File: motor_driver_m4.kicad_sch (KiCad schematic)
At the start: 32 parts, among them J13 Conn_01x01_Pin, J14 Conn_01x01_Pin, J15 Conn_01x01_Pin, M4 DRV8320SRTVR, Q19 NP80N06D6, Q20 NP80N06D6, Q21 NP80N06D6, Q22 NP80N06D6, Q23 NP80N06D6, Q24 NP80N06D6

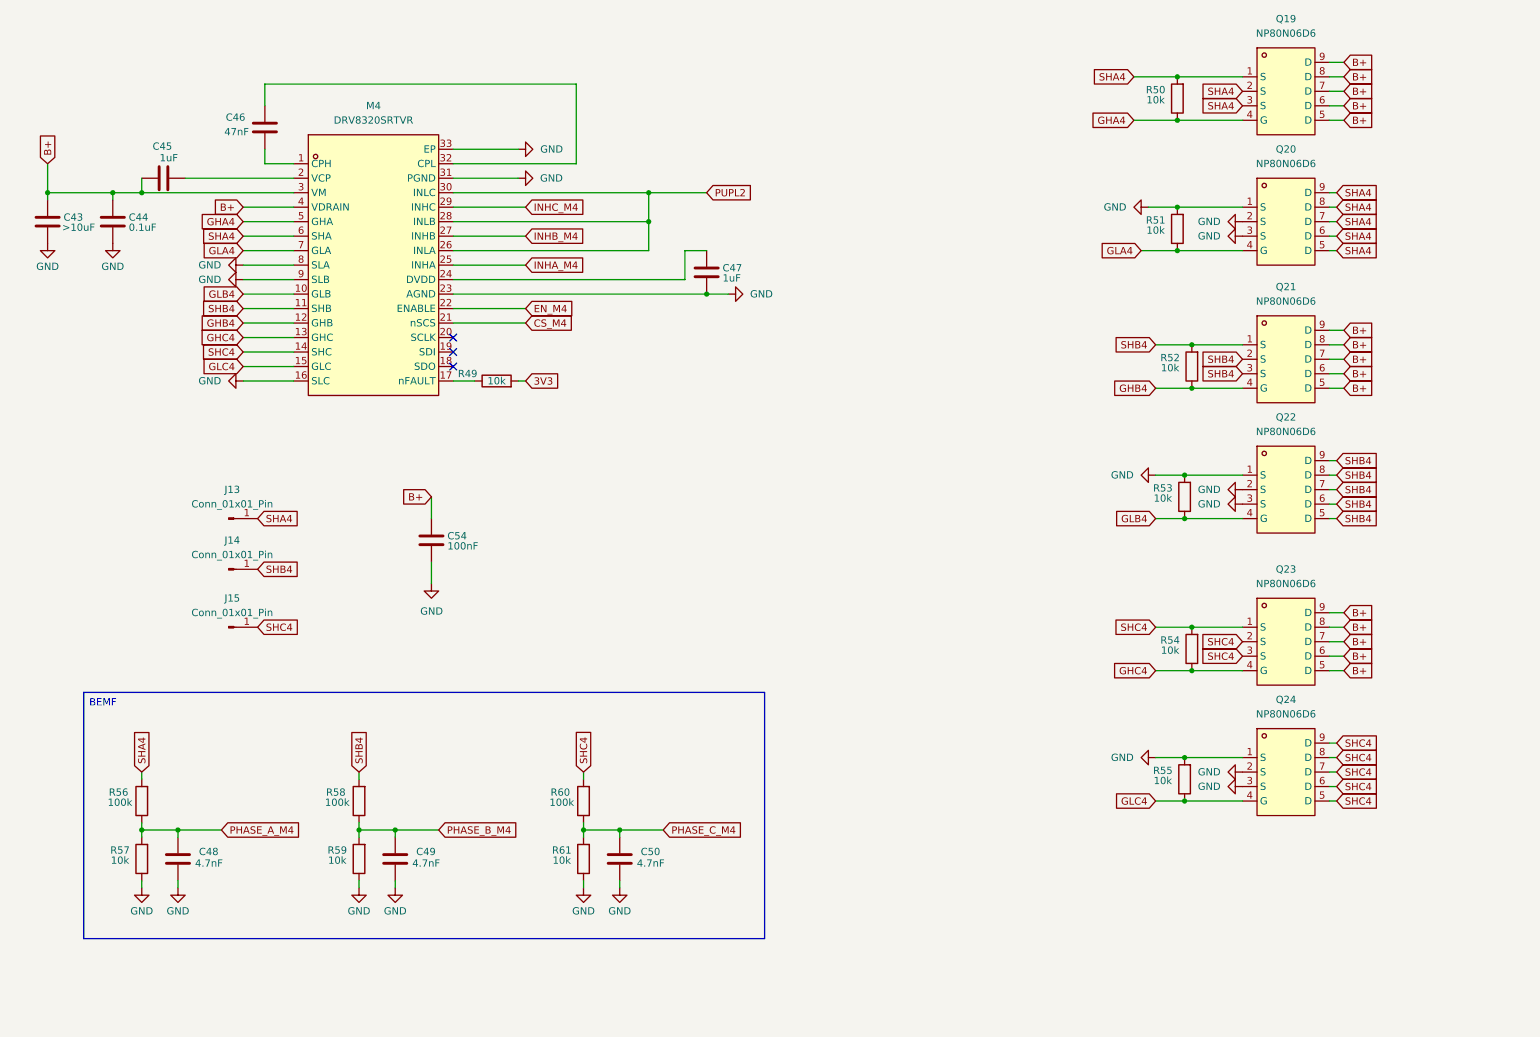
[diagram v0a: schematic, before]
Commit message: complete change in architecture,work in progress
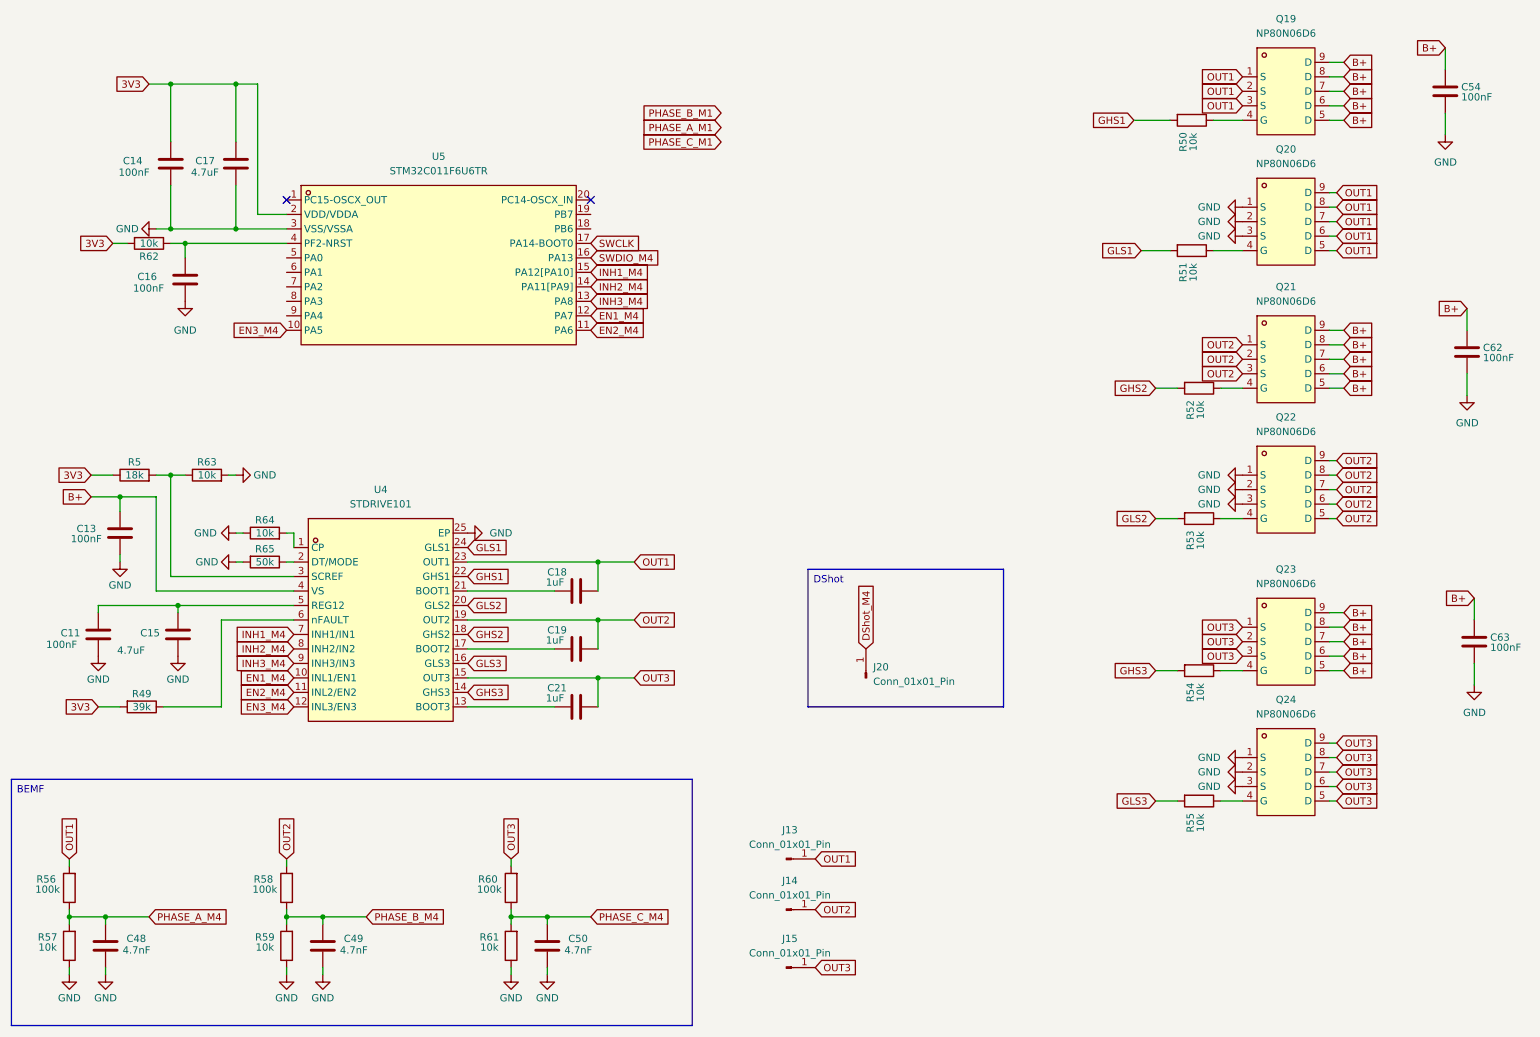
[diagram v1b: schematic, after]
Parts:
- removed C43: >10uF, easyeda2kicad:C0603, symbol Device:C
- removed C44: 0.1uF, easyeda2kicad:C0402, symbol Device:C
- removed C45, C47: 1uF, easyeda2kicad:C0603, symbol Device:C
- removed C46: 47nF, easyeda2kicad:C0603, symbol Device:C
- removed M4: DRV8320SRTVR, easyeda2kicad:WQFN-32_L5.0-W5.0-P0.50-TL-EP3.5, symbol easyeda2kicad:DRV8320SRTVR
- added C11, C62, C63: 100nF, easyeda2kicad:C0603, symbol Device:C
- added C13, C14, C16: 100nF, easyeda2kicad:C0402, symbol Device:C
- added C15: 4.7uF, easyeda2kicad:C0603, symbol Device:C
- added C17: 4.7uF, easyeda2kicad:C0402, symbol Device:C
- added C18, C19, C21: 1uF, easyeda2kicad:C0402, symbol Device:C
- added J20: Conn_01x01_Pin, deshan:Conn_1x1_small, symbol Connector:Conn_01x01_Pin
- added R5: 18k, easyeda2kicad:R0402, symbol Device:R
- added R62, R63, R64: 10k, easyeda2kicad:R0402, symbol Device:R
- added R65: 50k, easyeda2kicad:R0402, symbol Device:R
- added U4: STDRIVE101, easyeda2kicad:QFN-24_L4.0-W4.0-P0.50-BL-EP2.7, symbol easyeda2kicad:STDRIVE101
- added U5: STM32C011F6U6TR, easyeda2kicad:UFQFPN-20_L3.0-W3.0-P0.50-TL, symbol easyeda2kicad:STM32C011F6U6TR
- R49: value 10k -> 39k
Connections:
- net 3V3: now also C14.1, C17.1, R5.1, R62.2, U5.2 (VDD/VDDA)
- net B+: now also C13.1, C62.1, C63.1, U4.4 (VS)
- net GND: now also C11.2, C13.2, C14.2, C15.2, C16.2, C17.2, C62.2, C63.2, R63.2, R64.1, R65.2, U4.25 (EP), U5.3 (VSS/VSSA); no longer R51.2, R53.2, R55.2
- net at R49.1: now also U4.6 (nFAULT)
- net GHA4: no longer names the net of Q19.4 (G), R50.1
- net GHB4: no longer names the net of Q21.4 (G), R52.1
- net GHC4: no longer names the net of Q23.4 (G), R54.1
- net GLA4: no longer names the net of Q20.4 (G), R51.1
- net GLB4: no longer names the net of Q22.4 (G), R53.1
- net GLC4: no longer names the net of Q24.4 (G), R55.1
- net SHA4 renamed OUT1
- net OUT1: now also C18.1, U4.23 (OUT1); no longer R50.2
- net SHB4 renamed OUT2
- net OUT2: now also C19.1, U4.19 (OUT2); no longer R52.2
- net SHC4 renamed OUT3
- net OUT3: now also C21.1, U4.15 (OUT3); no longer R54.2
- new net: R65.1, U4.2 (DT/MODE)
- new net: C18.2, U4.21 (BOOT1)
- new net: C11.1, C15.1, U4.5 (REG12)
- new net: R64.2, U4.1 (CP)
- new net: C21.2, U4.13 (BOOT3)
- new net: C19.2, U4.17 (BOOT2)
- new net: R5.2, R63.1, U4.3 (SCREF)
- new net: C16.1, R62.1, U5.4 (PF2-NRST)
- new net DShot_M4: J20.1 (Pin_1)
- new net EN1_M4: U4.10 (INL1/EN1), U5.12 (PA7)
- new net EN2_M4: U4.11 (INL2/EN2), U5.11 (PA6)
- new net EN3_M4: U4.12 (INL3/EN3), U5.10 (PA5)
- new net GHS1: R50.2, U4.22 (GHS1)
- new net GHS2: R52.2, U4.18 (GHS2)
- new net GHS3: R54.2, U4.14 (GHS3)
- new net GLS1: R51.2, U4.24 (GLS1)
- new net GLS2: R53.2, U4.20 (GLS2)
- new net GLS3: R55.2, U4.16 (GLS3)
- new net INH1_M4: U4.7 (INH1/IN1), U5.15 (PA12[PA10])
- new net INH2_M4: U4.8 (INH2/IN2), U5.14 (PA11[PA9])
- new net INH3_M4: U4.9 (INH3/IN3), U5.13 (PA8)
- new net SWCLK: U5.17 (PA14-BOOT0)
- new net SWDIO_M4: U5.16 (PA13)
- no-connect marks 3 -> 2
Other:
- moved on the sheet: C48, C49, C50, C54, J13, J14, J15, R50, R51, R52, R53, R54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

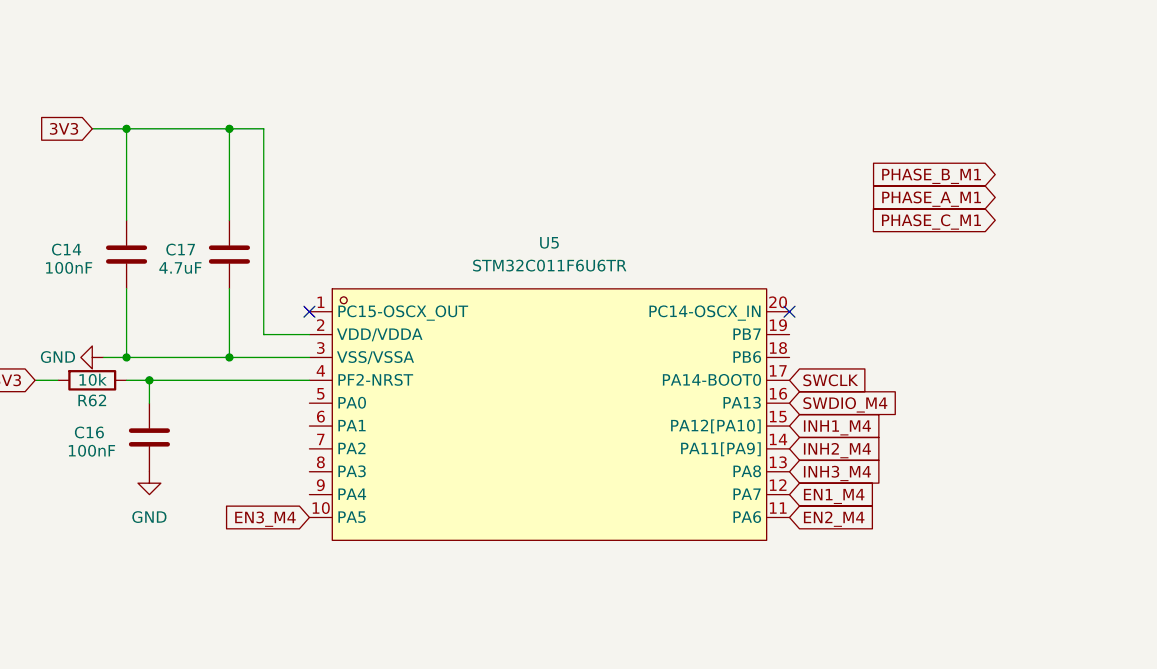
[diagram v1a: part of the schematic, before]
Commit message: ...
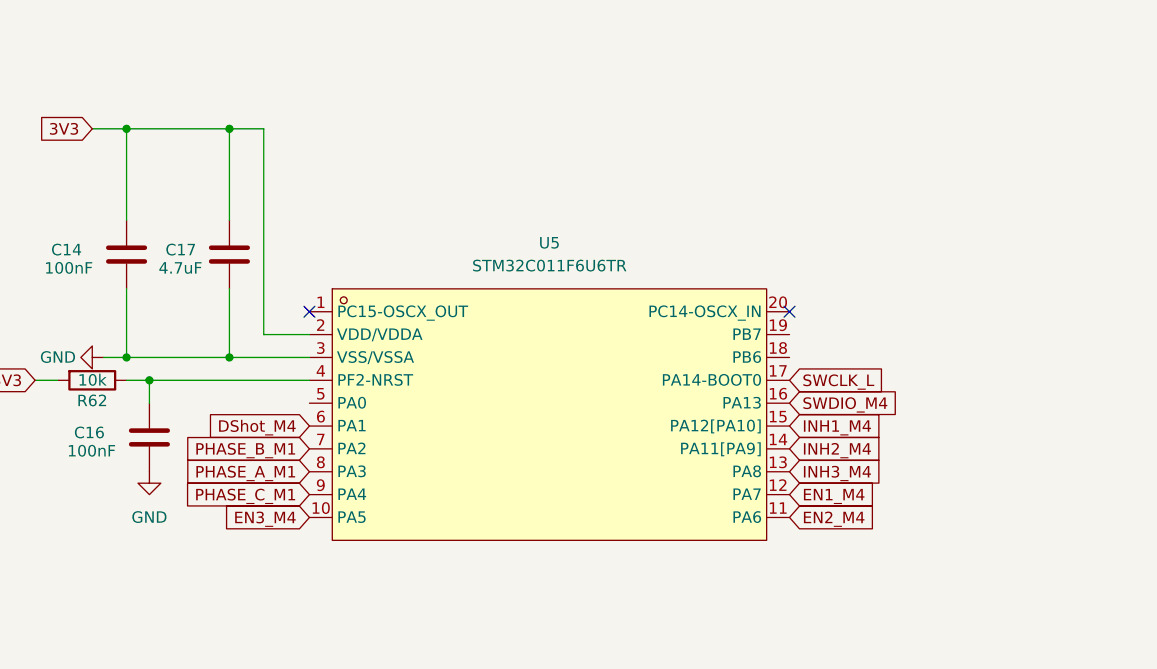
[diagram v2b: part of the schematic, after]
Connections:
- net DShot_M4: now also U5.6 (PA1)
- net PHASE_A_M1: now also U5.8 (PA3)
- net PHASE_B_M1: now also U5.7 (PA2)
- net PHASE_C_M1: now also U5.9 (PA4)
- net SWCLK renamed SWCLK_L
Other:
- title: (none) -> MOTOR DRIVER M4
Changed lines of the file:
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@@
 	(generator_version "10.0")
 	(paper "A4")
+	(title_block
+		(title "MOTOR DRIVER M4")
+		(rev "1.0")
+	)
 	(text_box "BEMF\n"
 		(exclude_from_sim no)
@@
 	(global_label "PHASE_C_M1"
 		(shape input)
-		(at 139.7 40.64 180)
+		(at 63.5 71.12 180)
 		(fields_autoplaced yes)
 		(effects
@@
 		)
 		(property "Intersheetrefs" "${INTERSHEET_REFS}"
-			(at 124.8011 40.64 0)
+			(at 48.6011 71.12 0)
 			(hide yes)
 			(show_name no)
@@
 	(global_label "PHASE_B_M1"
 		(shape input)
-		(at 139.7 35.56 180)
+		(at 63.5 66.04 180)
 		(fields_autoplaced yes)
 		(effects
@@
 		)
 		(property "Intersheetrefs" "${INTERSHEET_REFS}"
-			(at 124.8011 35.56 0)
+			(at 48.6011 66.04 0)
 			(hide yes)
 			(show_name no)
@@
 	(global_label "PHASE_A_M1"
 		(shape input)
-		(at 139.7 38.1 180)
+		(at 63.5 68.58 180)
 		(fields_autoplaced yes)
 		(effects
@@
 		)
 		(property "Intersheetrefs" "${INTERSHEET_REFS}"
-			(at 124.9825 38.1 0)
+			(at 48.7825 68.58 0)
 			(hide yes)
 			(show_name no)
@@
 		)
 	)
+	(global_label "DShot_M4"
+		(shape input)
+		(at 63.5 63.5 180)
+		(fields_autoplaced yes)
+		(effects
+			(font
+				(size 1.27 1.27)
+			)
+			(justify right)
+		)
+		(property "Intersheetrefs" "${INTERSHEET_REFS}"
+			(at 51.3831 63.5 0)
+			(hide yes)
+			(show_name no)
+			(do_not_autoplace no)
+			(effects
+				(font
+					(size 1.27 1.27)
+				)
+				(justify right)
+			)
+		)
+	)
 	(global_label "3V3"
 		(shape input)
@@
 		)
 	)
-	(global_label "SWCLK"
+	(global_label "SWCLK_L"
 		(shape input)
 		(at 116.84 58.42 0)
@@
 		)
 		(property "Intersheetrefs" "${INTERSHEET_REFS}"
-			(at 126.0542 58.42 0)
+			(at 128.0499 58.42 0)
 			(hide yes)
 			(show_name no)

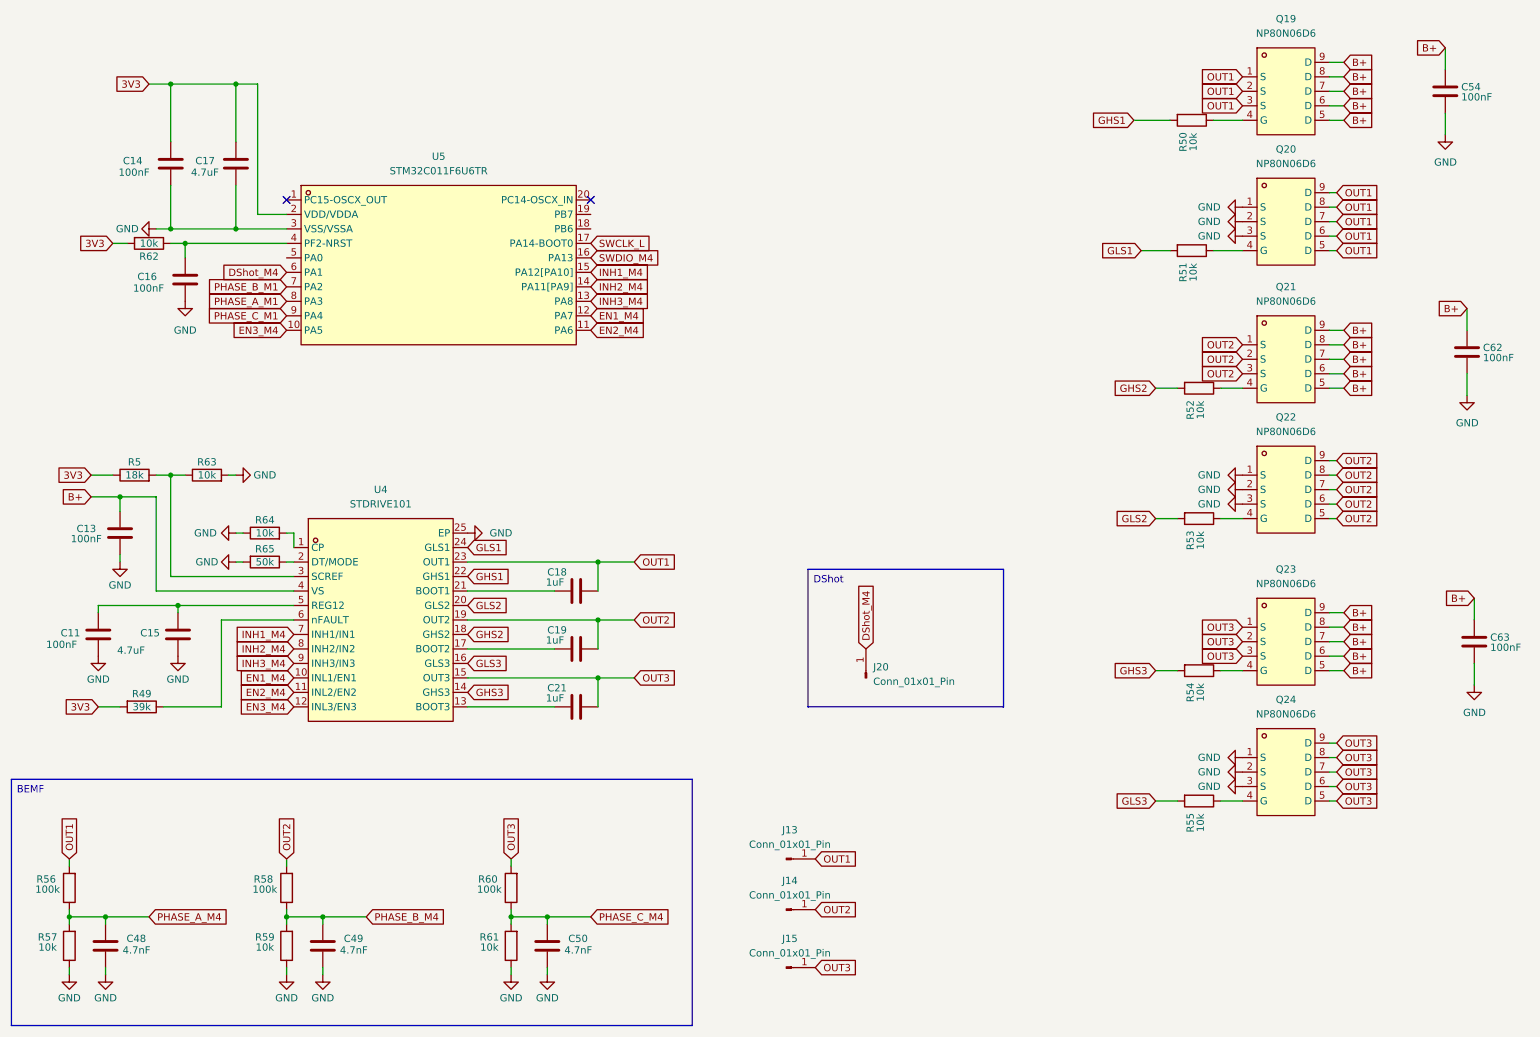
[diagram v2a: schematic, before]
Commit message: ...
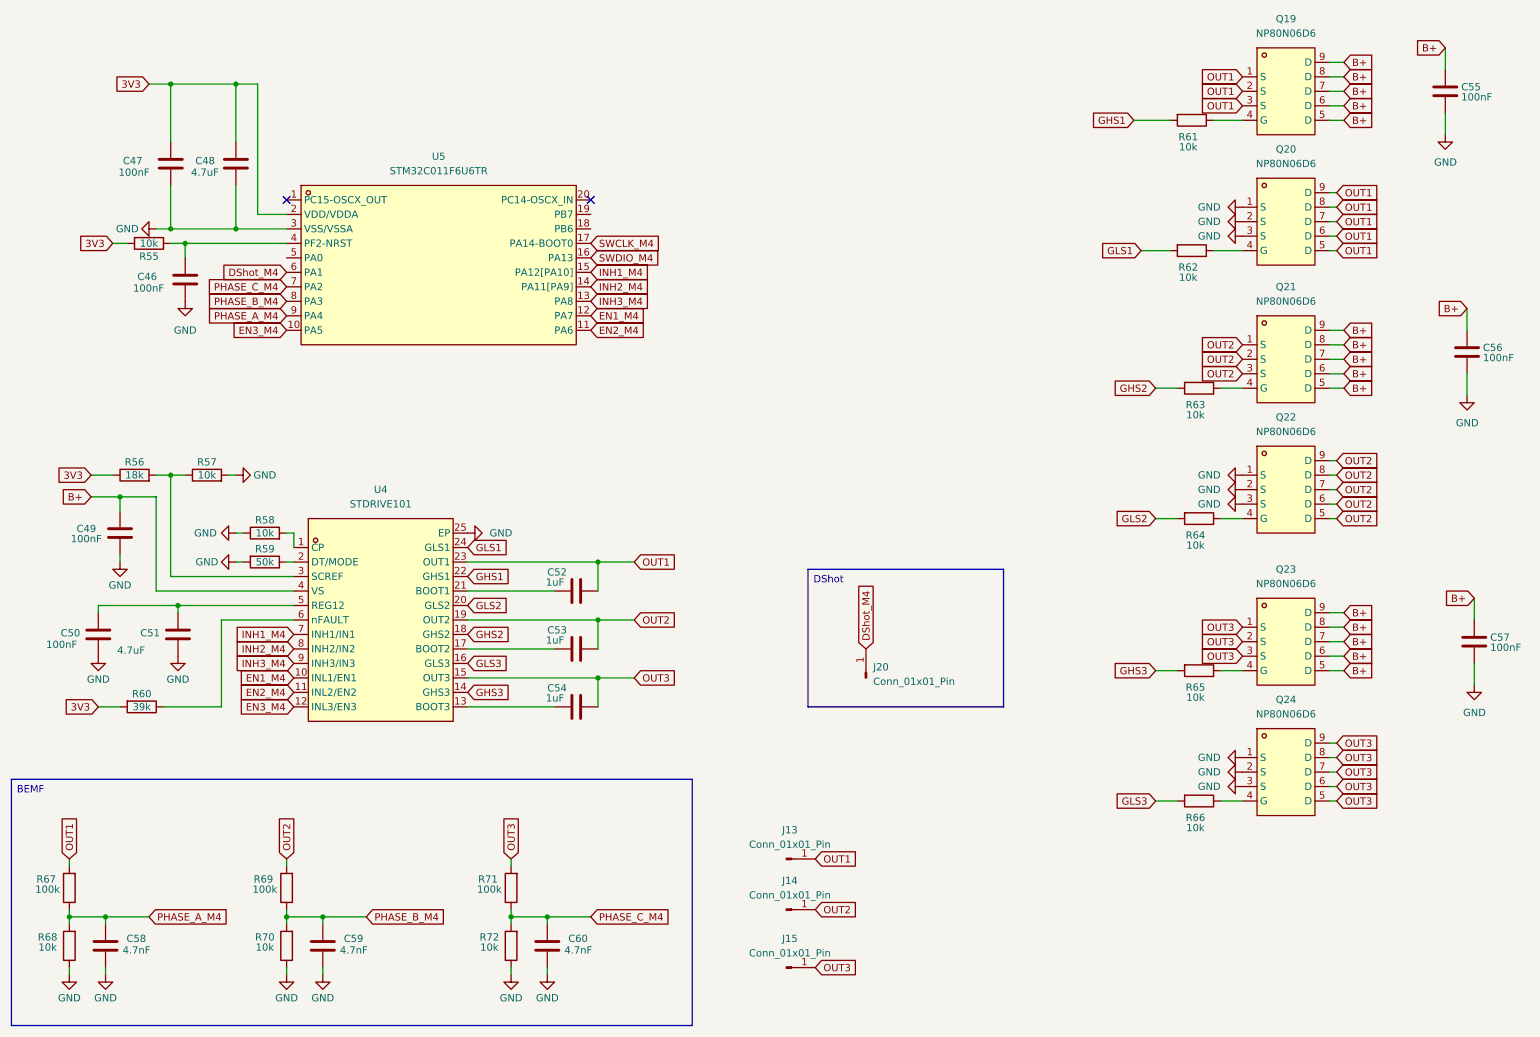
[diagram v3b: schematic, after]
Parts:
- J13, J14, J15: footprint deshan:Conn_1x1 -> deshan:Conn_01x01_Power
- J20: footprint deshan:Conn_1x1_small -> deshan:Conn_01x01_Pin
- renumbered C16 to C46, C14 to C47, C17 to C48, C13 to C49, C11 to C50, C15 to C51, C18 to C52, C19 to C53, C21 to C54, C54 to C55, C62 to C56, C63 to C57, C48 to C58, C49 to C59, C50 to C60, R62 to R55, R5 to R56, R63 to R57, R64 to R58, R65 to R59, R49 to R60, R50 to R61, R51 to R62, R52 to R63, R53 to R64, R54 to R65, R55 to R66, R56 to R67, R57 to R68, R58 to R69, R59 to R70, R60 to R71, R61 to R72
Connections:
- net PHASE_A_M1 is gone; now on net PHASE_B_M4: U5.8 (PA3)
- net PHASE_B_M1 is gone; now on net PHASE_C_M4: U5.7 (PA2)
- net PHASE_C_M1 is gone; now on net PHASE_A_M4: U5.9 (PA4)
- net SWCLK_L renamed SWCLK_M4
